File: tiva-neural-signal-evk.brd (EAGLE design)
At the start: 50.8 x 38.1 mm, 93 parts, among them IC1 TM4C123G, IC2 TLV70233, IC3 INA2332, IC4 OPA2320, IC5 OPA2320, IC6 INA2332, IC7 OPA2320, IC8 OPA2320, X1 USB, X2 MICROSD, Y1 16MHz, Y2 32.768kHz

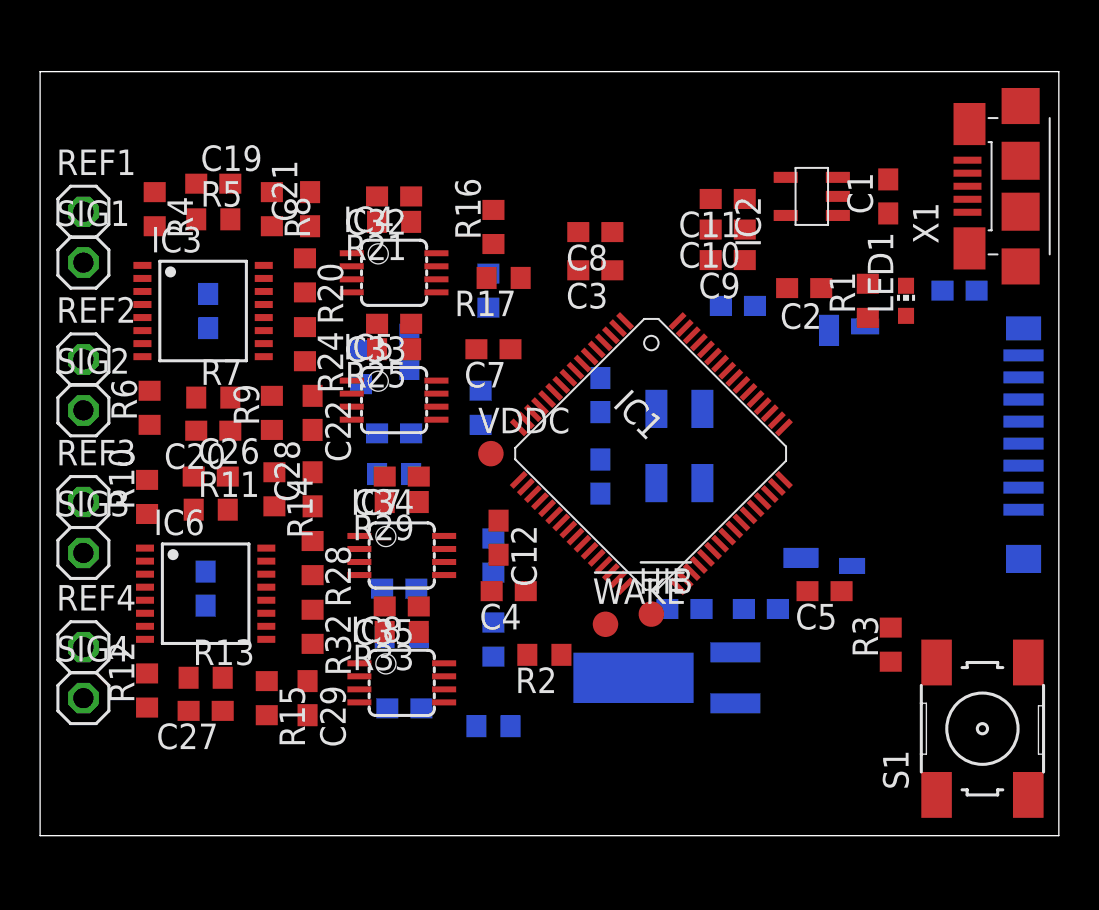
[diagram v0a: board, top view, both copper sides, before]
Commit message: Revert "Revert "added everything. initial routing complete with signal planes""
This reverts commit d55bffc2993c446258426b3721d1dfd936908fa6.
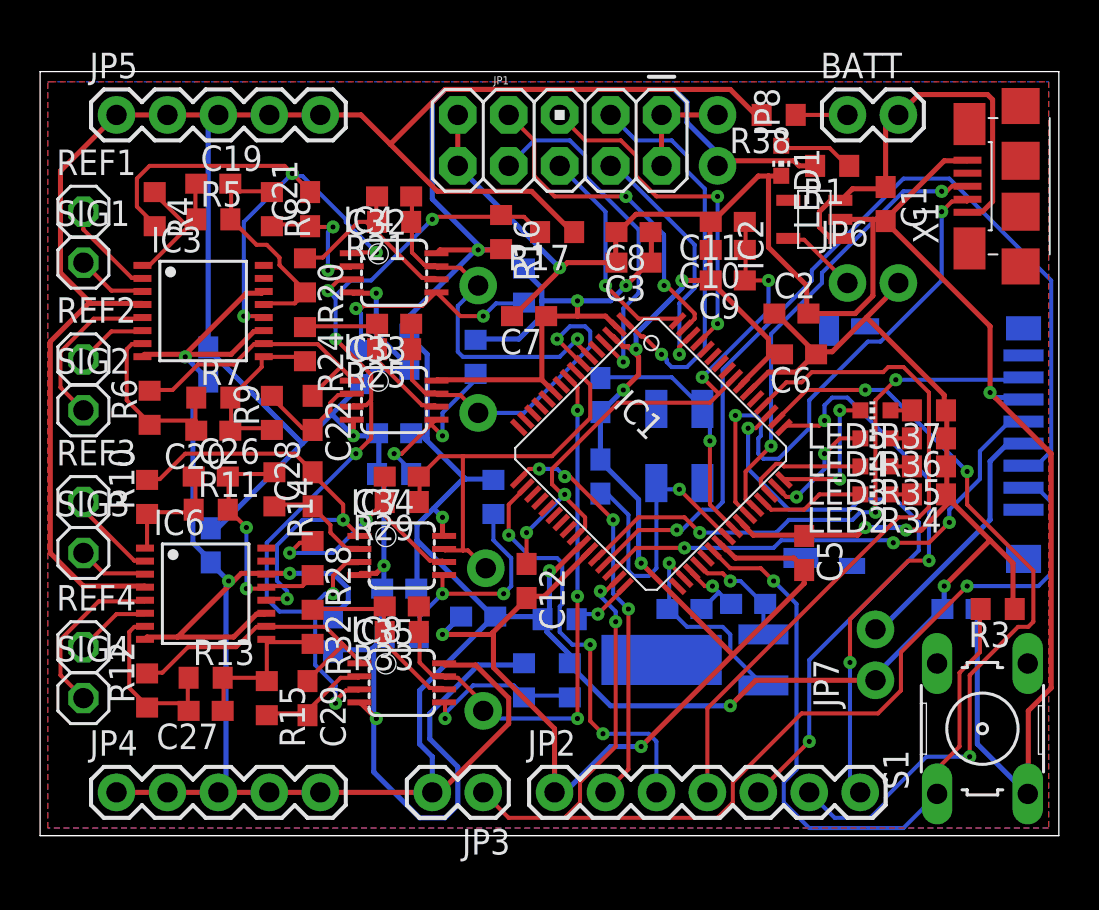
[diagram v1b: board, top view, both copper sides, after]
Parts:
- removed !HIB!, !WAKE!, VDDC: TPB1,27, testpad:B1,27
- added BATT, JP3: M02PTH, SparkFun-Connectors:1X02
- added CH1, CH2, CH3, CH4: M01NOSILK-KIT, SparkFun-Connectors:1X01NS-KIT
- added JP1: M05X2PTH, SparkFun-Connectors:AVR_ICSP
- added JP2: (no value), SparkFun-Connectors:1X07
- added JP4, JP5: (no value), SparkFun-Connectors:1X05
- added JP6, JP7, JP8: M021X02_NO_SILK, SparkFun-Connectors:1X02_NO_SILK
- added LED2, LED3, LED4, LED5: (no value), led:CHIP-LED0603
- added R34, R35, R36, R37: 330E, rcl:R0603
- added R38: 0E, rcl:R0603
- S1: device mor307:6MM_SWITCH -> CEDTv82:B3F-10XX
- moved C17 15.9 mm to (45.8, 11.3)
- moved LED1 9.35 mm to (37.0, 33.7), turned to 180 degrees
- moved R1 6.96 mm to (39.5, 33.4), turned to 180 degrees
- moved R3 5.62 mm to (47.8, 11.3), turned to 180 degrees
- moved C31 5.12 mm to (14.6, 10.0), turned to 270 degrees
- moved R30 4.44 mm to (26.4, 7.75), turned to 90 degrees
- moved C6 3.89 mm to (37.8, 24.0), flipped to the top, turned to 180 degrees
- moved R17 3.51 mm to (25.8, 30.1)
- moved R26 2.92 mm to (22.6, 16.9)
- moved C18 2.67 mm to (8.38, 23.5), turned to 90 degrees
- moved C12 2.57 mm to (24.3, 12.7)
- moved R22 2.55 mm to (21.7, 23.9)
- moved R31 2.54 mm to (24.1, 7.75)
- moved C7 2.43 mm to (24.4, 25.9)
- moved C25 2.17 mm to (8.51, 14.5), turned to 90 degrees
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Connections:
- new net AGND: C18.2, C23.2, C24.2, C25.2, C30.2, C31.2, IC3.4, IC4.4, IC5.4, IC6.4, IC7.4, IC8.4, JP5.1, JP5.2, JP5.3, JP5.4, JP5.5, R17.1, R19.1, R23.1, R27.1, R31.1, R38.2
- new net N$31: LED2.A, R34.2
- new net N$35: LED3.A, R35.2
- new net N$36: LED4.A, R36.2
- new net N$37: LED5.A, R37.2
- new net N$38: IC2.5, JP6.1
- new net N$39: BATT.1, R38.1
- new net N$40: JP7.2, X2.4
- new net N$41: JP1.1, JP1.2, JP8.1
- net !HIB!: no longer !HIB!.TP
- net !RESET!: now also S1.1; no longer S1.3, S1.4
- net !WAKE!: no longer !WAKE!.TP
- net +3V3: now also JP3.2, JP4.1, JP4.2, JP4.3, JP4.4, JP4.5, JP6.2, JP7.1, JP8.2, R34.1, R35.1, R36.1, R37.1; no longer IC2.5, X2.4
- net GND: now also JP1.10, JP1.9, JP2.1, S1.3; no longer C18.2, C23.2, C24.2, C25.2, C30.2, C31.2, IC3.4, IC4.4, IC5.4, IC6.4, IC7.4, IC8.4, R17.1, R19.1, R23.1, R27.1, R31.1, S1.1, S1.2
- net PA0: now also JP2.2
- net PA1: now also JP2.3
- net PB0: now also LED2.C
- net PB1: now also LED3.C
- net PB2: now also LED4.C
- net PB3: now also LED5.C
- net PB6: now also JP1.3
- net PB7: now also JP1.8
- net PC0: now also JP2.4
- net PC1: now also JP2.5
- net PC2: now also JP2.6
- net PC3: now also JP2.7
- net PD0: now also JP1.5
- net PD1: now also JP1.4
- net PD2: now also JP1.7
- net PD3: now also JP1.6
- net PE0: now also CH4.1
- net PE1: now also CH3.1
- net PE2: now also CH2.1
- net PE3: now also CH1.1
- net PF3: now also JP3.1
- net VBUS: now also BATT.2
- net VDDC: no longer VDDC.TP
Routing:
- net +3V3: track 0.00 -> 265.3 mm, vias 0 -> 12
- net GND: track 0.00 -> 174.4 mm, vias 0 -> 8
- net AGND: track 0.00 -> 158.2 mm, vias 0 -> 4
- net PF3: track 0.00 -> 54.6 mm, vias 0 -> 3
- net PF1: track 0.00 -> 46.7 mm, vias 0 -> 1
- net VREF: track 0.00 -> 46.4 mm, vias 0 -> 6
- net PC2: track 0.00 -> 39.0 mm, vias 0 -> 3
- net PC0: track 0.00 -> 34.7 mm
- net !RESET!: track 0.00 -> 34.5 mm, vias 0 -> 1
- net VDDC: track 0.00 -> 31.1 mm, vias 0 -> 4
- net PC1: track 0.00 -> 30.2 mm, vias 0 -> 2
- net PE0: track 0.00 -> 29.3 mm, vias 0 -> 3
- net PF0: track 0.00 -> 29.0 mm, vias 0 -> 3
- net N$5: track 0.00 -> 28.5 mm, vias 0 -> 3
- net PC3: track 0.00 -> 28.0 mm, vias 0 -> 3
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- added copper zone on layer 16, net AGND
- added copper zone on layer 1, net GND

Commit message: Revert "added everything. initial routing complete with signal planes"
This reverts commit afc261f9183dc80193b5e18bad7752eddb98d99b.
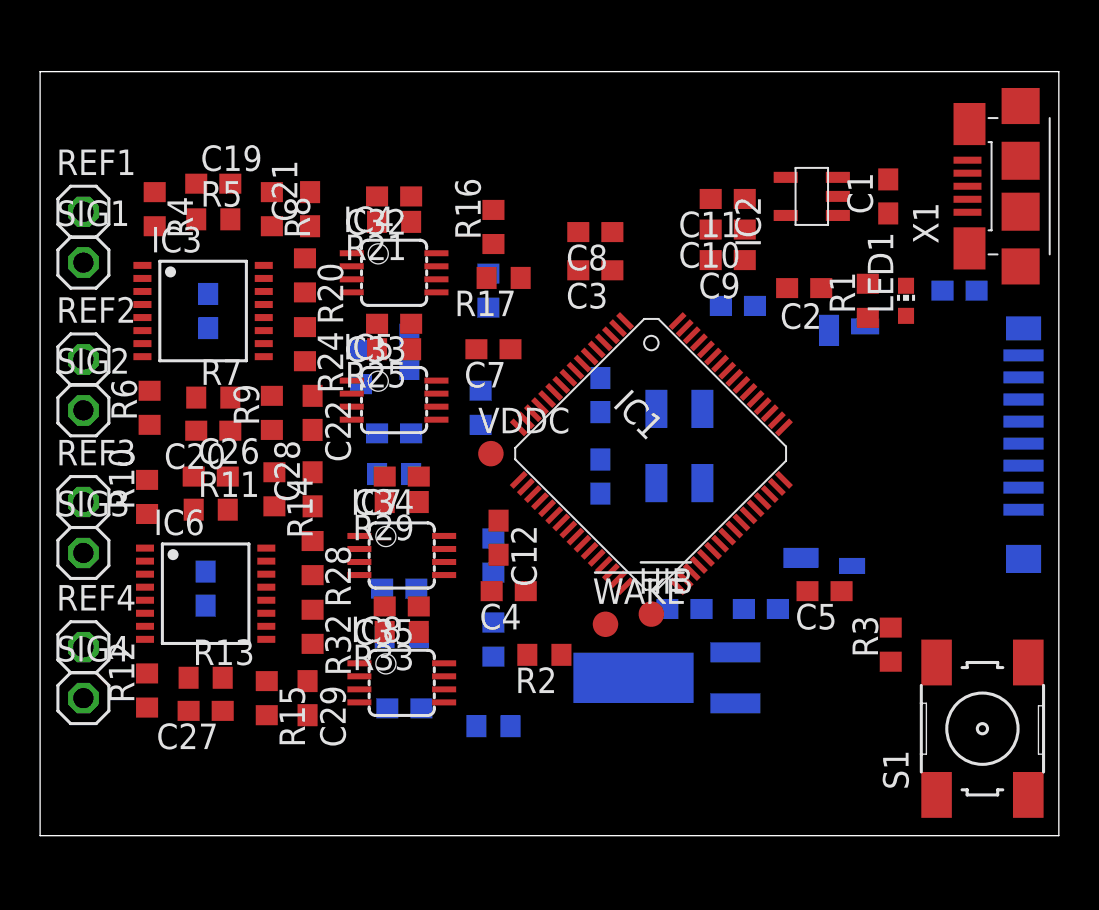
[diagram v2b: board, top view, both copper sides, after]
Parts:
- removed BATT, JP3: M02PTH, SparkFun-Connectors:1X02
- removed CH1, CH2, CH3, CH4: M01NOSILK-KIT, SparkFun-Connectors:1X01NS-KIT
- removed JP1: M05X2PTH, SparkFun-Connectors:AVR_ICSP
- removed JP2: (no value), SparkFun-Connectors:1X07
- removed JP4, JP5: (no value), SparkFun-Connectors:1X05
- removed JP6, JP7, JP8: M021X02_NO_SILK, SparkFun-Connectors:1X02_NO_SILK
- removed LED2, LED3, LED4, LED5: (no value), led:CHIP-LED0603
- removed R34, R35, R36, R37: 330E, rcl:R0603
- removed R38: 0E, rcl:R0603
- added !HIB!, !WAKE!, VDDC: TPB1,27, testpad:B1,27
- S1: device CEDTv82:B3F-10XX -> mor307:6MM_SWITCH
- moved C17 15.9 mm to (45.8, 27.2)
- moved LED1 9.35 mm to (43.2, 26.7), turned to 0 degrees
- moved R1 6.96 mm to (41.3, 26.7), turned to 90 degrees
- moved R3 5.62 mm to (42.4, 9.53), turned to 90 degrees
- moved C31 5.12 mm to (18.2, 6.35), turned to 0 degrees
- moved R30 4.44 mm to (22.6, 5.46), turned to 0 degrees
- moved C6 3.89 mm to (34.8, 26.4), flipped to the bottom, turned to 0 degrees
- moved R17 3.51 mm to (23.1, 27.8)
- moved R26 2.92 mm to (22.6, 14.0)
- moved C18 2.67 mm to (8.38, 26.2), turned to 270 degrees
- moved C12 2.57 mm to (22.9, 14.9)
- moved R22 2.55 mm to (22.0, 21.3)
- moved R31 2.54 mm to (22.6, 9.78)
- moved C7 2.43 mm to (22.6, 24.3)
- moved C25 2.17 mm to (8.26, 12.3), turned to 270 degrees
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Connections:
- removed net AGND: C18.2, C23.2, C24.2, C25.2, C30.2, C31.2, IC3.4, IC4.4, IC5.4, IC6.4, IC7.4, IC8.4, JP5.1, JP5.2, JP5.3, JP5.4, JP5.5, R17.1, R19.1, R23.1, R27.1, R31.1, R38.2
- removed net N$31: LED2.A, R34.2
- removed net N$35: LED3.A, R35.2
- removed net N$36: LED4.A, R36.2
- removed net N$37: LED5.A, R37.2
- removed net N$38: IC2.5, JP6.1
- removed net N$39: BATT.1, R38.1
- removed net N$40: JP7.2, X2.4
- removed net N$41: JP1.1, JP1.2, JP8.1
- net !HIB!: now also !HIB!.TP
- net !RESET!: now also S1.3, S1.4; no longer S1.1
- net !WAKE!: now also !WAKE!.TP
- net +3V3: now also IC2.5, X2.4; no longer JP3.2, JP4.1, JP4.2, JP4.3, JP4.4, JP4.5, JP6.2, JP7.1, JP8.2, R34.1, R35.1, R36.1, R37.1
- net GND: now also C18.2, C23.2, C24.2, C25.2, C30.2, C31.2, IC3.4, IC4.4, IC5.4, IC6.4, IC7.4, IC8.4, R17.1, R19.1, R23.1, R27.1, R31.1, S1.1, S1.2; no longer JP1.10, JP1.9, JP2.1, S1.3
- net PA0: no longer JP2.2
- net PA1: no longer JP2.3
- net PB0: no longer LED2.C
- net PB1: no longer LED3.C
- net PB2: no longer LED4.C
- net PB3: no longer LED5.C
- net PB6: no longer JP1.3
- net PB7: no longer JP1.8
- net PC0: no longer JP2.4
- net PC1: no longer JP2.5
- net PC2: no longer JP2.6
- net PC3: no longer JP2.7
- net PD0: no longer JP1.5
- net PD1: no longer JP1.4
- net PD2: no longer JP1.7
- net PD3: no longer JP1.6
- net PE0: no longer CH4.1
- net PE1: no longer CH3.1
- net PE2: no longer CH2.1
- net PE3: no longer CH1.1
- net PF3: no longer JP3.1
- net VBUS: no longer BATT.2
- net VDDC: now also VDDC.TP
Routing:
- net +3V3: track 265.3 -> 0.00 mm, vias 12 -> 0
- net GND: track 174.4 -> 0.00 mm, vias 8 -> 0
- net AGND: track 158.2 -> 0.00 mm, vias 4 -> 0
- net PF3: track 54.6 -> 0.00 mm, vias 3 -> 0
- net PF1: track 46.7 -> 0.00 mm, vias 1 -> 0
- net VREF: track 46.4 -> 0.00 mm, vias 6 -> 0
- net PC2: track 39.0 -> 0.00 mm, vias 3 -> 0
- net PC0: track 34.7 -> 0.00 mm
- net !RESET!: track 34.5 -> 0.00 mm, vias 1 -> 0
- net VDDC: track 31.1 -> 0.00 mm, vias 4 -> 0
- net PC1: track 30.2 -> 0.00 mm, vias 2 -> 0
- net PE0: track 29.3 -> 0.00 mm, vias 3 -> 0
- net PF0: track 29.0 -> 0.00 mm, vias 3 -> 0
- net N$5: track 28.5 -> 0.00 mm, vias 3 -> 0
- net PC3: track 28.0 -> 0.00 mm, vias 3 -> 0
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- removed copper zone on layer 16, net AGND
- removed copper zone on layer 1, net GND
